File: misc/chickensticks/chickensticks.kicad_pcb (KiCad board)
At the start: 4 copper layers, 42 x 100 mm, 102 parts, among them J1 Conn_01x05_Pin, J10 Conn_01x03_Pin, J2 HRO_TYPE-C-31-M-12, J3 Conn_01x04, J4 Conn_01x06, J5 Conn_01x06, J6 Conn_01x04, J7 Conn_01x04, J8 S02-25200300, J9 SMA, Q1 Si2371EDS, Q2 DMG9926UDM, Q3 2N7002, SW1 SKRPANE010, SW2 EC11E18244AU, U1 USBLC6-2SC6, U2 STM32L433CCTx, U3 TJA1042T-3, U4 LR2021IMLTRT, U5 LP5907MFX-3.3, U6 MCP73831-2-MC, U7 BQ29700, Y1 25 MHz, Y2 TG2520SMN 32.0000M-MCGNNM0

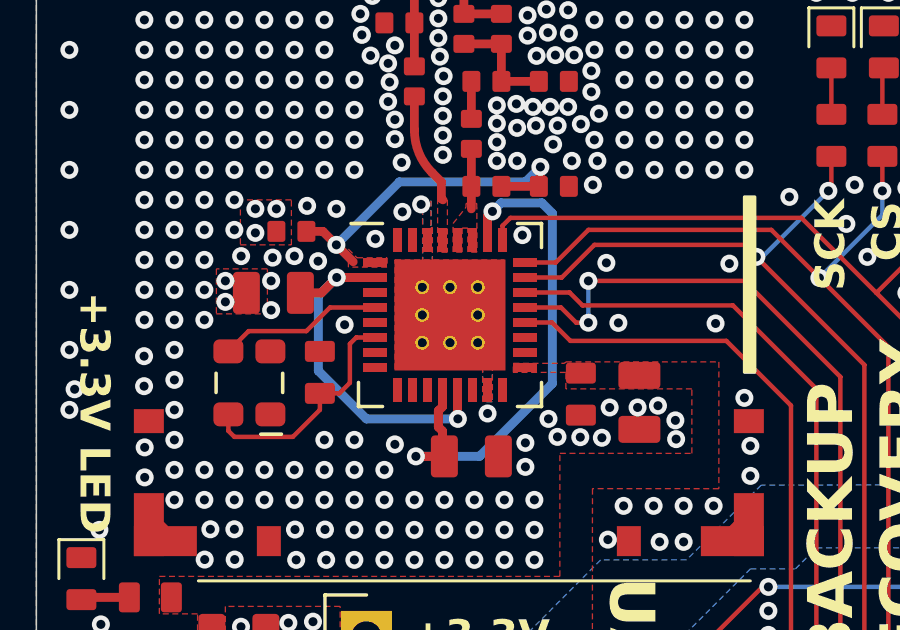
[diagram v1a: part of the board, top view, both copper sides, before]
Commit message: Begin prep for second board review
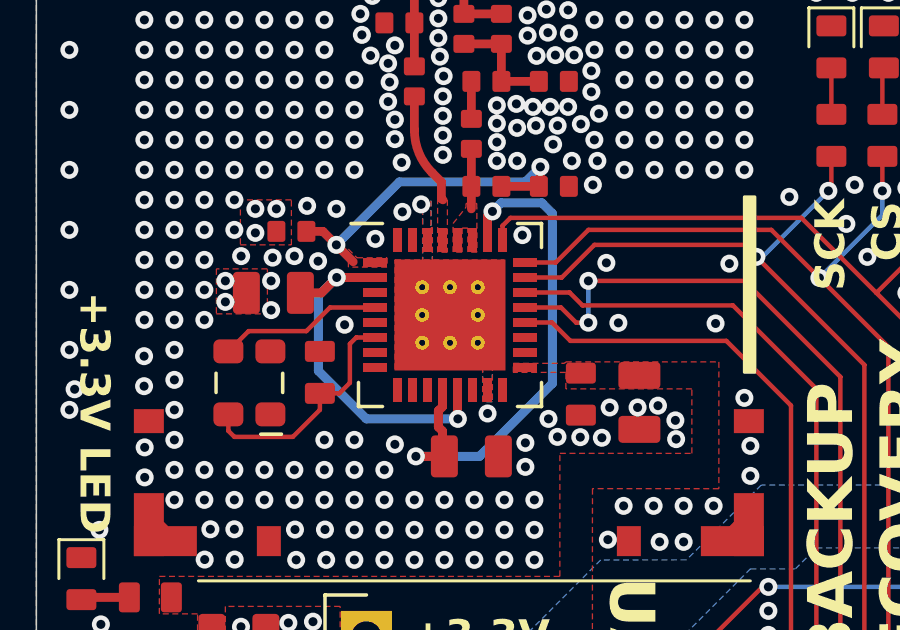
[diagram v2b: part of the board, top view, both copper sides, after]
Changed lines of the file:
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@@
 			(at -0.925 -0.925)
 			(size 0.4625 0.4625)
-			(drill 0.3)
+			(drill 0.2)
 			(property pad_prop_heatsink)
 			(layers "*.Cu" "*.Mask")
@@
 			(at -0.925 0)
 			(size 0.4625 0.4625)
-			(drill 0.3)
+			(drill 0.2)
 			(property pad_prop_heatsink)
 			(layers "*.Cu" "*.Mask")
@@
 			(at -0.925 0.925)
 			(size 0.4625 0.4625)
-			(drill 0.3)
+			(drill 0.2)
 			(property pad_prop_heatsink)
 			(layers "*.Cu" "*.Mask")
@@
 			(at 0 -0.925)
 			(size 0.4625 0.4625)
-			(drill 0.3)
+			(drill 0.2)
 			(property pad_prop_heatsink)
 			(layers "*.Cu" "*.Mask")
@@
 			(at 0 0.925)
 			(size 0.4625 0.4625)
-			(drill 0.3)
+			(drill 0.2)
 			(property pad_prop_heatsink)
 			(layers "*.Cu" "*.Mask")
@@
 			(at 0.925 -0.925)
 			(size 0.4625 0.4625)
-			(drill 0.3)
+			(drill 0.2)
 			(property pad_prop_heatsink)
 			(layers "*.Cu" "*.Mask")
@@
 			(at 0.925 0)
 			(size 0.4625 0.4625)
-			(drill 0.3)
+			(drill 0.2)
 			(property pad_prop_heatsink)
 			(layers "*.Cu" "*.Mask")
@@
 			(at 0.925 0.925)
 			(size 0.4625 0.4625)
-			(drill 0.3)
+			(drill 0.2)
 			(property pad_prop_heatsink)
 			(layers "*.Cu" "*.Mask")
